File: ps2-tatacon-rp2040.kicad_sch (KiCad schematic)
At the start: 15 parts, among them J1 Buttons, J2 Right, J3 Left, J4 Center, U1 RP2040-Zero

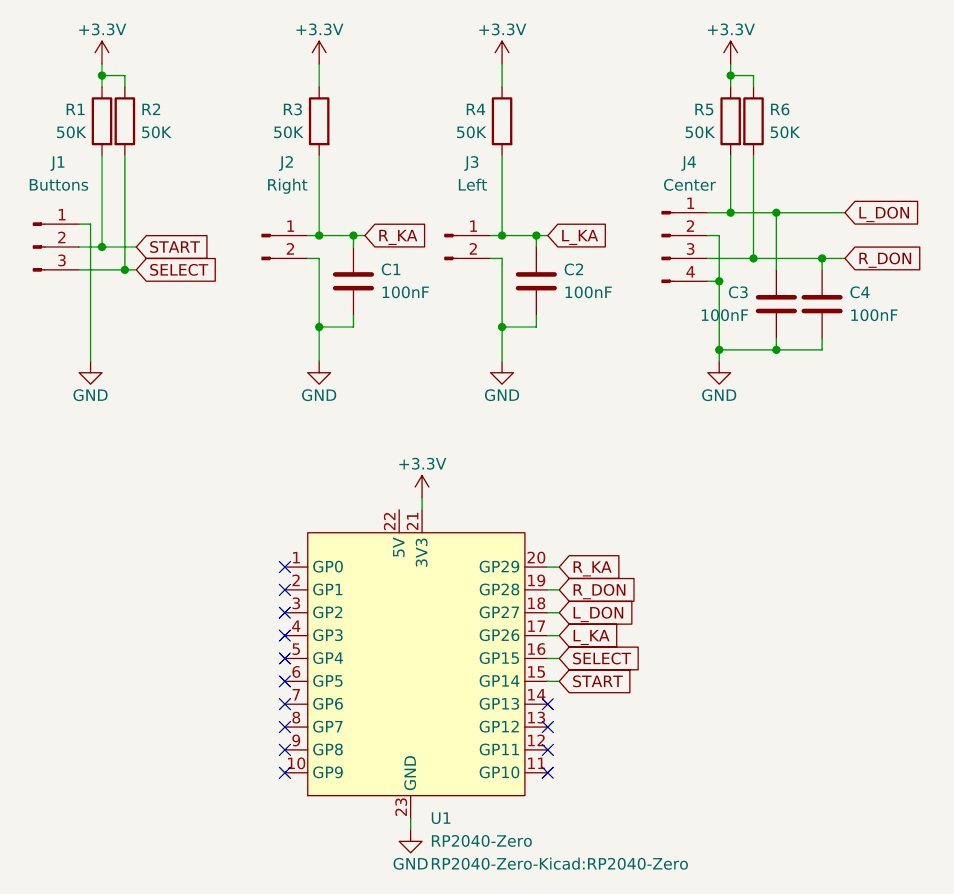
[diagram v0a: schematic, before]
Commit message: First revision finished
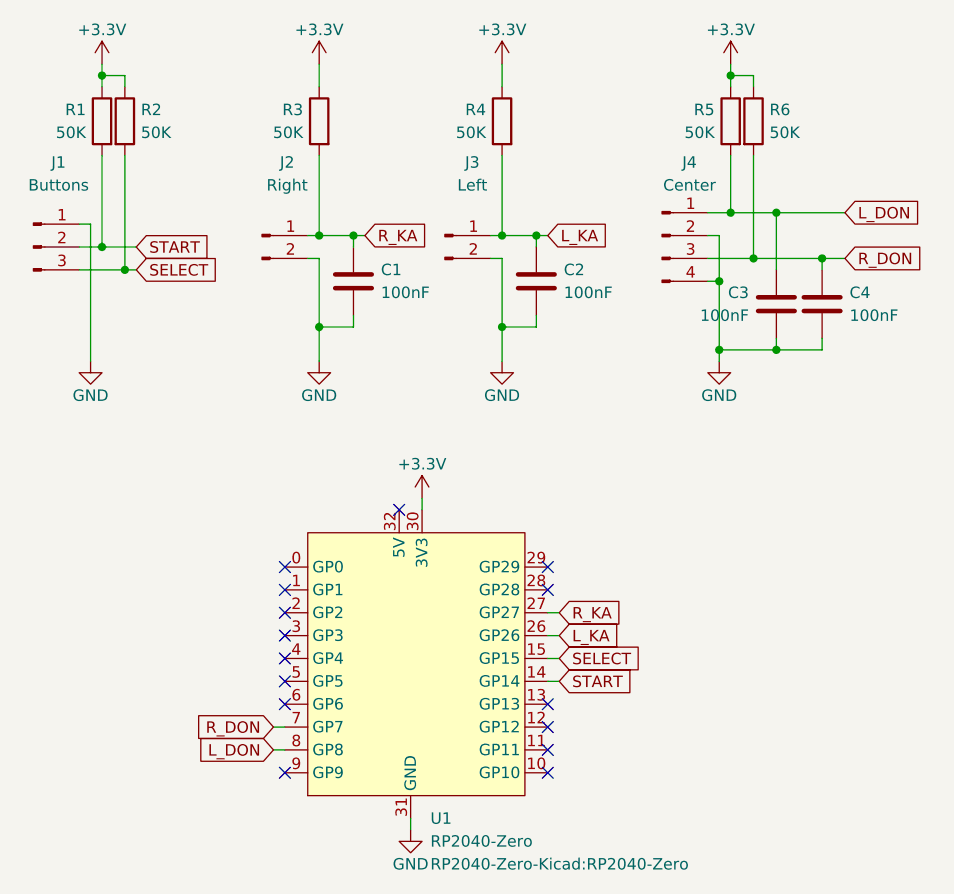
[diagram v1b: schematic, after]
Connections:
- net +3.3V: now also U1.30 (3V3); no longer U1.21 (3V3)
- net GND: now also U1.31 (GND); no longer U1.23 (GND)
- net L_DON: now also U1.8 (GP8); no longer U1.18 (GP27)
- net L_KA: now also U1.26 (GP26); no longer U1.17 (GP26)
- net R_DON: now also U1.7 (GP7); no longer U1.19 (GP28)
- net R_KA: now also U1.27 (GP27); no longer U1.20 (GP29)
- net SELECT: now also U1.15 (GP15); no longer U1.16 (GP15)
- net START: now also U1.14 (GP14); no longer U1.15 (GP14)
- no-connect marks 14 -> 15
